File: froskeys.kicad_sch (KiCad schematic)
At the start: 25 parts, among them SW1 MX, SW10 RotaryEncoder_Switch, SW2 MX, SW3 MX, SW4 MX, SW5 MX, SW6 MX, SW7 MX, SW8 MX, SW9 MX, U1 XIAO-RP2040-DIP, U2 OLED

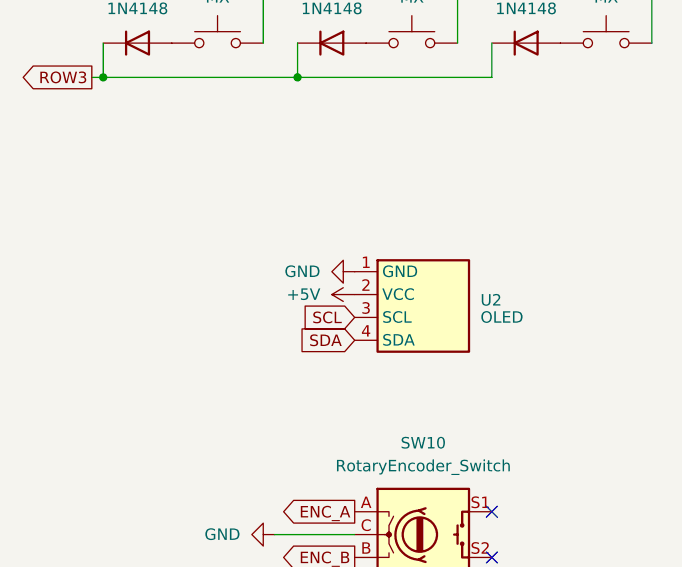
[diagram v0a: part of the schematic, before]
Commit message: Optimise
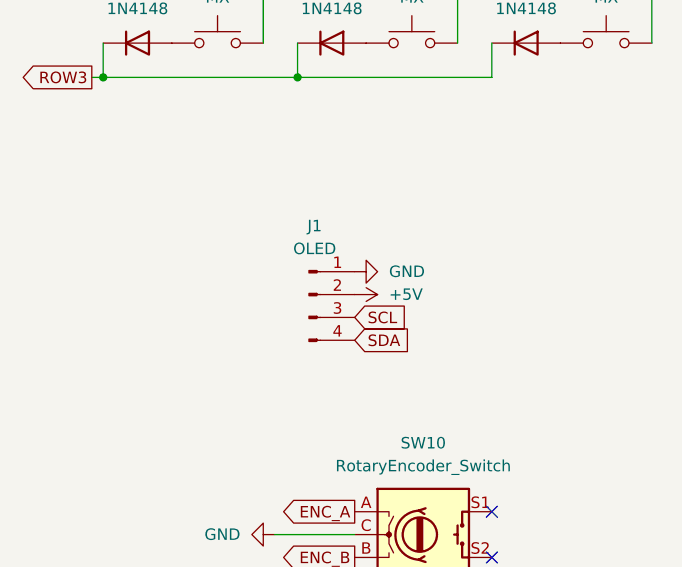
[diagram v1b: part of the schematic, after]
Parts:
- removed U2: OLED, OLED:SSD1306-0.91-OLED-4pin-128x32, symbol OLED:0.91{dblquote}_128x32_I2C_OLED_Display
- added J1: OLED, OLED:SSD1306-0.91-OLED-4pin-128x32, symbol Connector:Conn_01x04_Pin
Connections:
- net +5V: now also J1.2 (Pin_2)
- net GND: now also J1.1 (Pin_1)
- net SCL: now also J1.3 (Pin_3)
- net SDA: now also J1.4 (Pin_4)
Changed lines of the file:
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@@
 	(global_label "SDA"
 		(shape input)
-		(at 208.28 118.11 180)
+		(at 208.28 118.11 0)
 		(fields_autoplaced yes)
 		(effects
@@
 				(size 1.27 1.27)
 			)
-			(justify right)
+			(justify left)
 		)
 		(property "Intersheetrefs" "${INTERSHEET_REFS}"
-			(at 201.7267 118.11 0)
-			(effects
-				(font
-					(size 1.27 1.27)
-				)
-				(justify right)
+			(at 214.8333 118.11 0)
+			(effects
+				(font
+					(size 1.27 1.27)
+				)
+				(justify left)
 				(hide yes)
 			)
@@
 	(global_label "SCL"
 		(shape input)
-		(at 208.28 115.57 180)
+		(at 208.28 115.57 0)
 		(fields_autoplaced yes)
 		(effects
@@
 				(size 1.27 1.27)
 			)
-			(justify right)
+			(justify left)
 		)
 		(property "Intersheetrefs" "${INTERSHEET_REFS}"
-			(at 201.7872 115.57 0)
-			(effects
-				(font
-					(size 1.27 1.27)
-				)
-				(justify right)
+			(at 214.7728 115.57 0)
+			(effects
+				(font
+					(size 1.27 1.27)
+				)
+				(justify left)
 				(hide yes)
 			)
@@
 	(symbol
 		(lib_id "power:GND")
-		(at 208.28 110.49 270)
+		(at 208.28 110.49 90)
 		(unit 1)
 		(exclude_from_sim no)
@@
 		(fields_autoplaced yes)
 		(property "Reference" "#PWR03"
-			(at 201.93 110.49 0)
+			(at 214.63 110.49 0)
 			(effects
 				(font
@@
 		)
 		(property "Value" "GND"
-			(at 204.47 110.4899 90)
+			(at 212.09 110.4899 90)
 			(effects
 				(font
@@
 	)
 	(symbol
+		(lib_id "Connector:Conn_01x04_Pin")
+		(at 203.2 113.03 0)
+		(unit 1)
+		(exclude_from_sim no)
+		(in_bom yes)
+		(on_board yes)
+		(dnp no)
+		(fields_autoplaced yes)
+		(property "Reference" "J1"
+			(at 203.835 105.41 0)
+			(effects
+				(font
+					(size 1.27 1.27)
+				)
+			)
+		)
+		(property "Value" "OLED"
+			(at 203.835 107.95 0)
+			(effects
+				(font
+					(size 1.27 1.27)
+				)
+			)
+		)
+		(property "Footprint" "OLED:SSD1306-0.91-OLED-4pin-128x32"
+			(at 203.2 113.03 0)
+			(effects
+				(font
+					(size 1.27 1.27)
+				)
+				(hide yes)
+			)
+		)
+		(property "Datasheet" "~"
+			(at 203.2 113.03 0)
+			(effects
+				(font
+					(size 1.27 1.27)
+				)
+				(hide yes)
+			)
+		)
+		(property "Description" "Generic connector, single row, 01x04, script generated"
+			(at 203.2 113.03 0)
+			(effects
+				(font
+					(size 1.27 1.27)
+				)
+				(hide yes)
+			)
+		)
+		(pin "2"
+		)
+		(pin "1"
+		)
+		(pin "3"
+		)
+		(pin "4"
+		)
+		(instances
+			(project ""
+				(path "/7f4b6218-3a01-4dd6-a14f-3aa125e7c41a"
+					(reference "J1")
+					(unit 1)
+				)
+			)
+		)
+	)
+	(symbol
 		(lib_id "Diode:1N4148")
 		(at 227.33 71.12 0)
@@
 	(symbol
 		(lib_id "power:+5V")
-		(at 208.28 113.03 90)
+		(at 208.28 113.03 270)
 		(unit 1)
 		(exclude_from_sim no)
@@
 		(fields_autoplaced yes)
 		(property "Reference" "#PWR04"
-			(at 212.09 113.03 0)
+			(at 204.47 113.03 0)
 			(effects
 				(font
@@
 		)
 		(property "Value" "+5V"
-			(at 204.47 113.0299 90)
+			(at 212.09 113.0299 90)
 			(effects
 				(font
@@
 					(unit 1)
 				)
-			)
-		)
-	)
-	(symbol
-		(lib_id "OLED:0.91{dblquote}_128x32_I2C_OLED_Display")
-		(at 215.9 114.3 0)
-		(unit 1)
-		(exclude_from_sim no)
-		(in_bom yes)
-		(on_board yes)
-		(dnp no)
-		(fields_autoplaced yes)
-		(property "Reference" "U2"
-			(at 222.25 113.6649 0)
-			(effects
-				(font
-					(size 1.27 1.27)
-				)
-				(justify left)
-			)
-		)
-		(property "Value" "OLED"
-			(at 222.25 115.57 0)
-			(effects
-				(font
-					(size 1.27 1.27)
-				)
-				(justify left)
-			)
-		)
-		(property "Footprint" "OLED:SSD1306-0.91-OLED-4pin-128x32"
-			(at 215.9 114.3 0)
-			(effects
-				(font
-					(size 1.27 1.27)
-				)
-				(hide yes)
-			)
-		)
-		(property "Datasheet" ""
-			(at 215.9 114.3 0)
-			(effects
-				(font
-					(size 1.27 1.27)
-				)
-				(hide yes)
-			)
-		)
-		(property "Description" ""
-			(at 215.9 114.3 0)
-			(effects
-				(font
-					(size 1.27 1.27)
-				)
-				(hide yes)
-			)
-		)
-		(pin "3"
-		)
-		(pin "4"
-		)
-		(pin "2"
-		)
-		(pin "1"
-		)
-		(instances
-			(project ""
-				(path "/7f4b6218-3a01-4dd6-a14f-3aa125e7c41a"
-					(reference "U2")
-					(unit 1)
-				)
